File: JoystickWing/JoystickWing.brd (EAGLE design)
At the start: 32.7 x 69.8 mm, 21 parts, among them J1 5747844-4

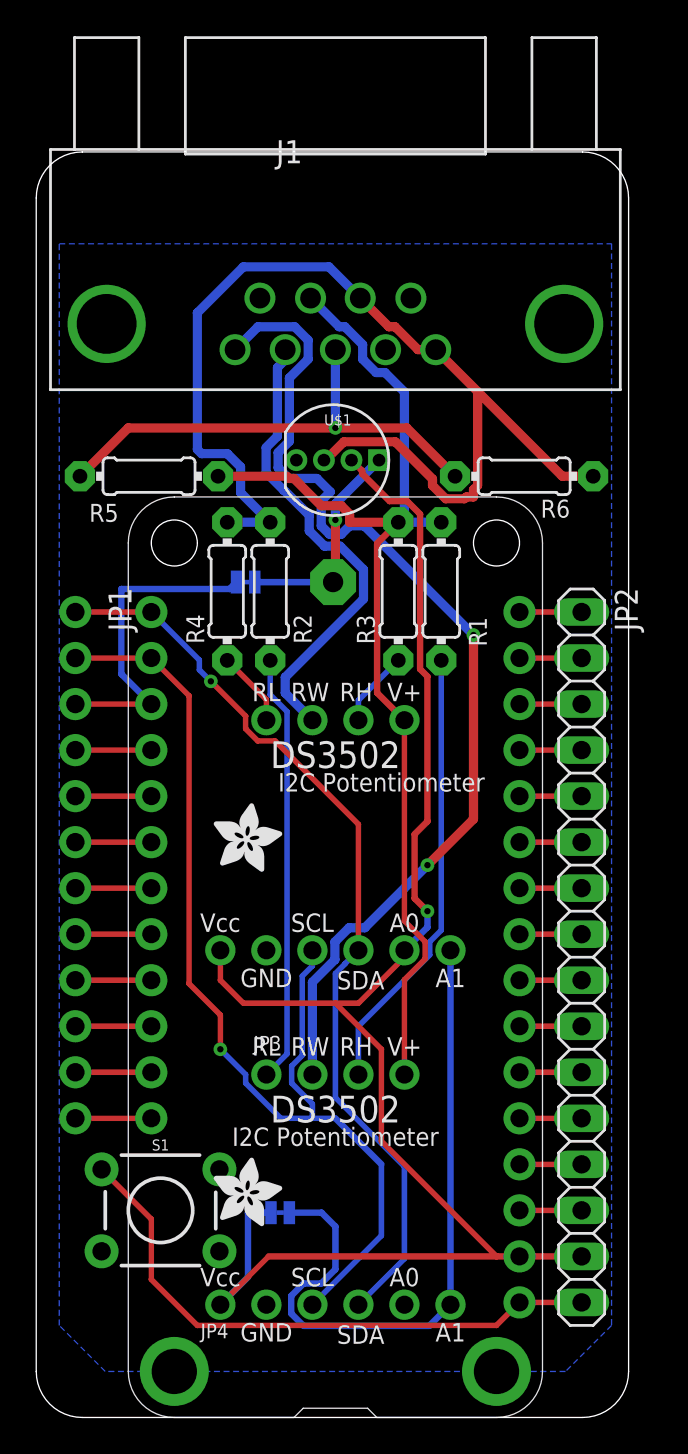
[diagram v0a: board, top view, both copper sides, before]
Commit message: Added the missing Neopixel led pads and updated the switch to DTS-3: 3.5x6mm style switch.
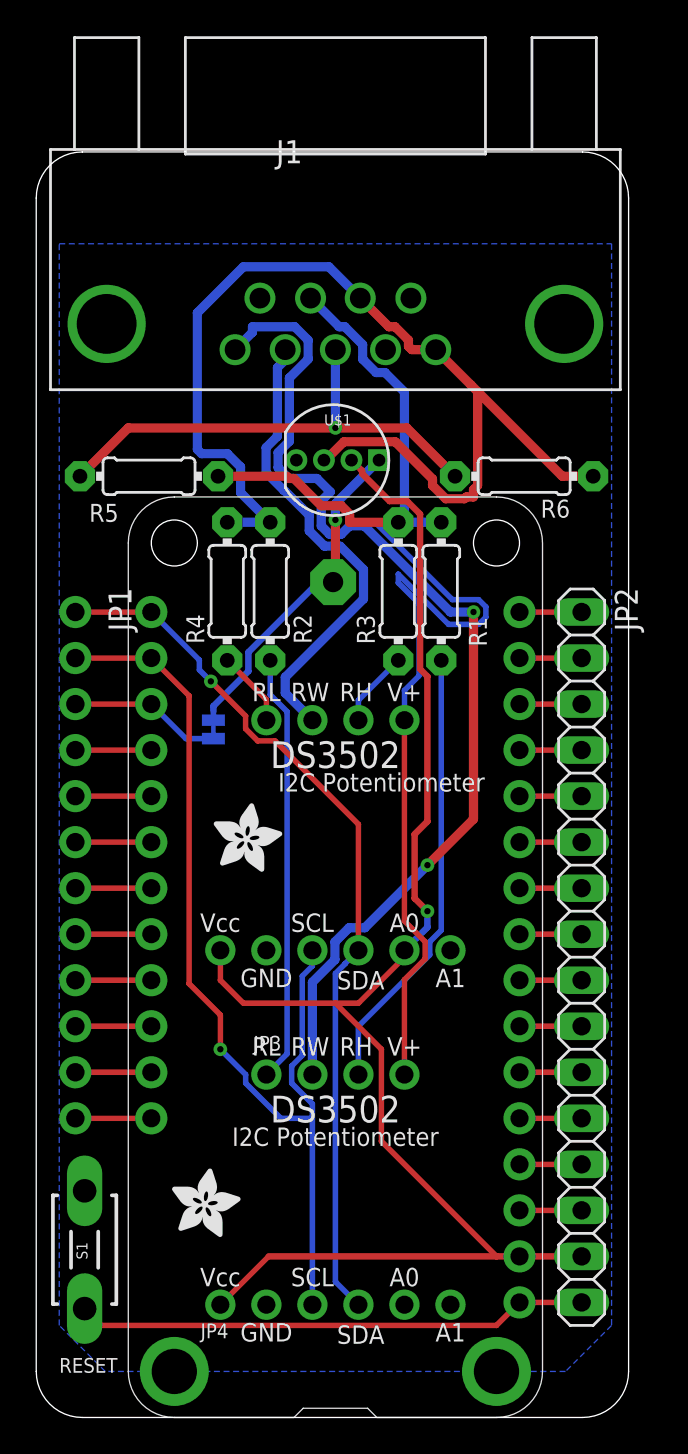
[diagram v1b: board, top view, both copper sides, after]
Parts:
- removed A1: JUMPER-SMT_2_NC_TRACE_SILK, SparkFun-Jumpers:SMT-JUMPER_2_NC_TRACE_SILK
- S1: value MOMENTARY-SWITCH-SPST-PTH-6.0MM -> RESET; device SparkFun-Switches:TACTILE_SWITCH_PTH_6.0MM -> milador:DTS-3
- moved JP7 8.32 mm to (9.78, 38.0), turned to 90 degrees
- moved S1 4.72 mm to (2.67, 9.26), turned to 90 degrees
- moved U$10 2.38 mm to (7.48, 9.94)
- renumbered NEOPIN to PAD1
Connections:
- removed net ADDR: A1.1, JP4.6, JP6.6
- new net P1A1: JP4.6
- new net P2A1: JP6.6
- net GND: now also S1.2, U$1.P3; no longer S1.3, U$1.3
- net N$25: now also U$1.P1; no longer U$1.1
- net VCC: now also U$1.P2; no longer A1.2, U$1.2
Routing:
- net ADDR: track 38.6 -> 0.00 mm
- net +12V: track 61.3 -> 74.2 mm
- net N$1: track 17.7 -> 8.41 mm
- net VCC: track 89.9 -> 82.9 mm
- net N$25: track 12.1 -> 18.6 mm
- net N$24: track 32.5 -> 28.3 mm
- net SCL: track 58.7 -> 54.8 mm
- net SDA: track 50.9 -> 48.8 mm
- net P1RW: track 57.8 -> 58.8 mm
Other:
- board text removed: "3V"
- board text removed: "JoyStick"
- board text removed: "Uncut = 1 Cut = 0"

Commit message: Revert "Added the missing Neopixel led pads and updated the switch to DTS-3: 3.5x6mm style switch."
This reverts commit 7139ee0b9ca13871835c94f32c5504dad1631a27.
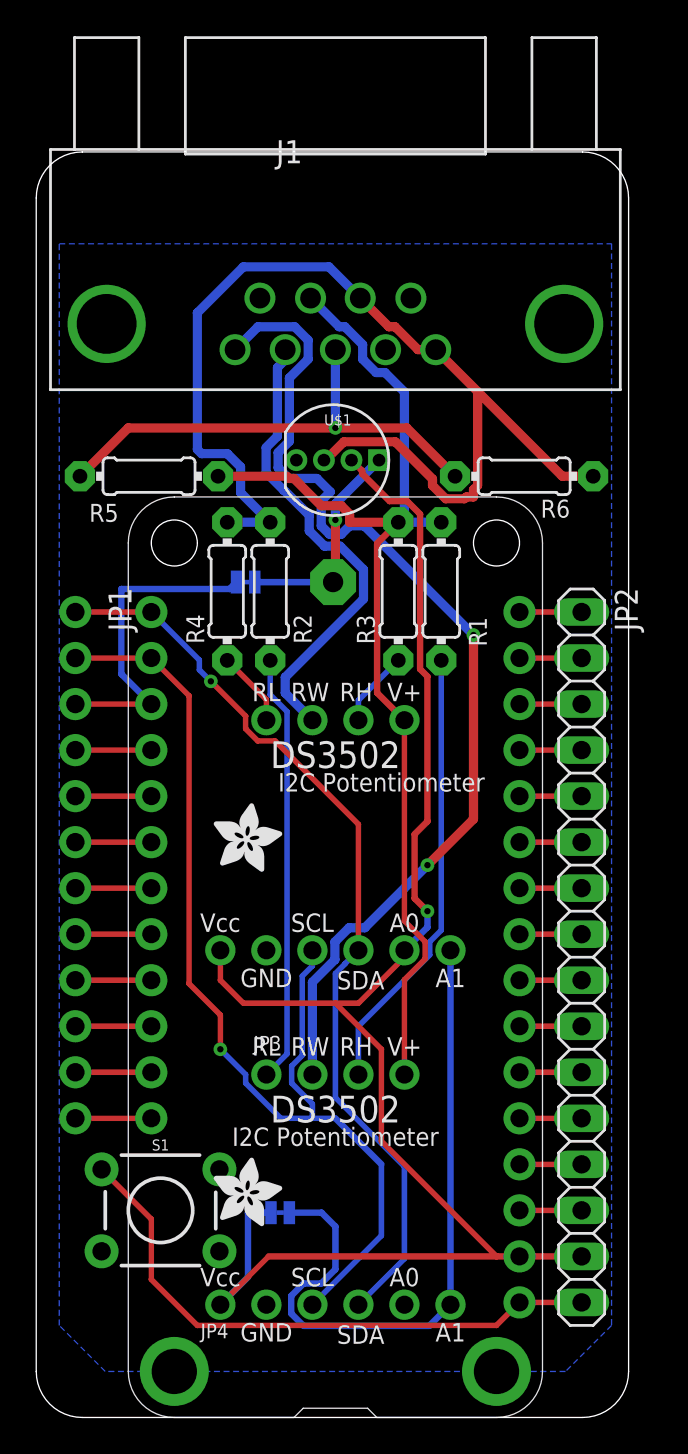
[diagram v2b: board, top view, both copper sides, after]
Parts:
- added A1: JUMPER-SMT_2_NC_TRACE_SILK, SparkFun-Jumpers:SMT-JUMPER_2_NC_TRACE_SILK
- S1: value RESET -> MOMENTARY-SWITCH-SPST-PTH-6.0MM; device milador:DTS-3 -> SparkFun-Switches:TACTILE_SWITCH_PTH_6.0MM
- moved JP7 8.32 mm to (11.6, 46.1), turned to 180 degrees
- moved S1 4.72 mm to (6.86, 11.4), turned to 0 degrees
- moved U$10 2.38 mm to (9.78, 10.5)
- renumbered PAD1 to NEOPIN
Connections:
- removed net P1A1: JP4.6
- removed net P2A1: JP6.6
- new net ADDR: A1.1, JP4.6, JP6.6
- net GND: now also S1.3, U$1.3; no longer S1.2, U$1.P3
- net N$25: now also U$1.1; no longer U$1.P1
- net VCC: now also A1.2, U$1.2; no longer U$1.P2
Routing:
- net ADDR: track 0.00 -> 38.6 mm
- net +12V: track 74.2 -> 61.3 mm
- net N$1: track 8.41 -> 17.7 mm
- net VCC: track 82.9 -> 89.9 mm
- net N$25: track 18.6 -> 12.1 mm
- net N$24: track 28.3 -> 32.5 mm
- net SCL: track 54.8 -> 58.7 mm
- net SDA: track 48.8 -> 50.9 mm
- net P1RW: track 58.8 -> 57.8 mm
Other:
- board text added: "3V"
- board text added: "JoyStick"
- board text added: "Uncut = 1 Cut = 0"
